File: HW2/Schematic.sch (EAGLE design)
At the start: 3 parts

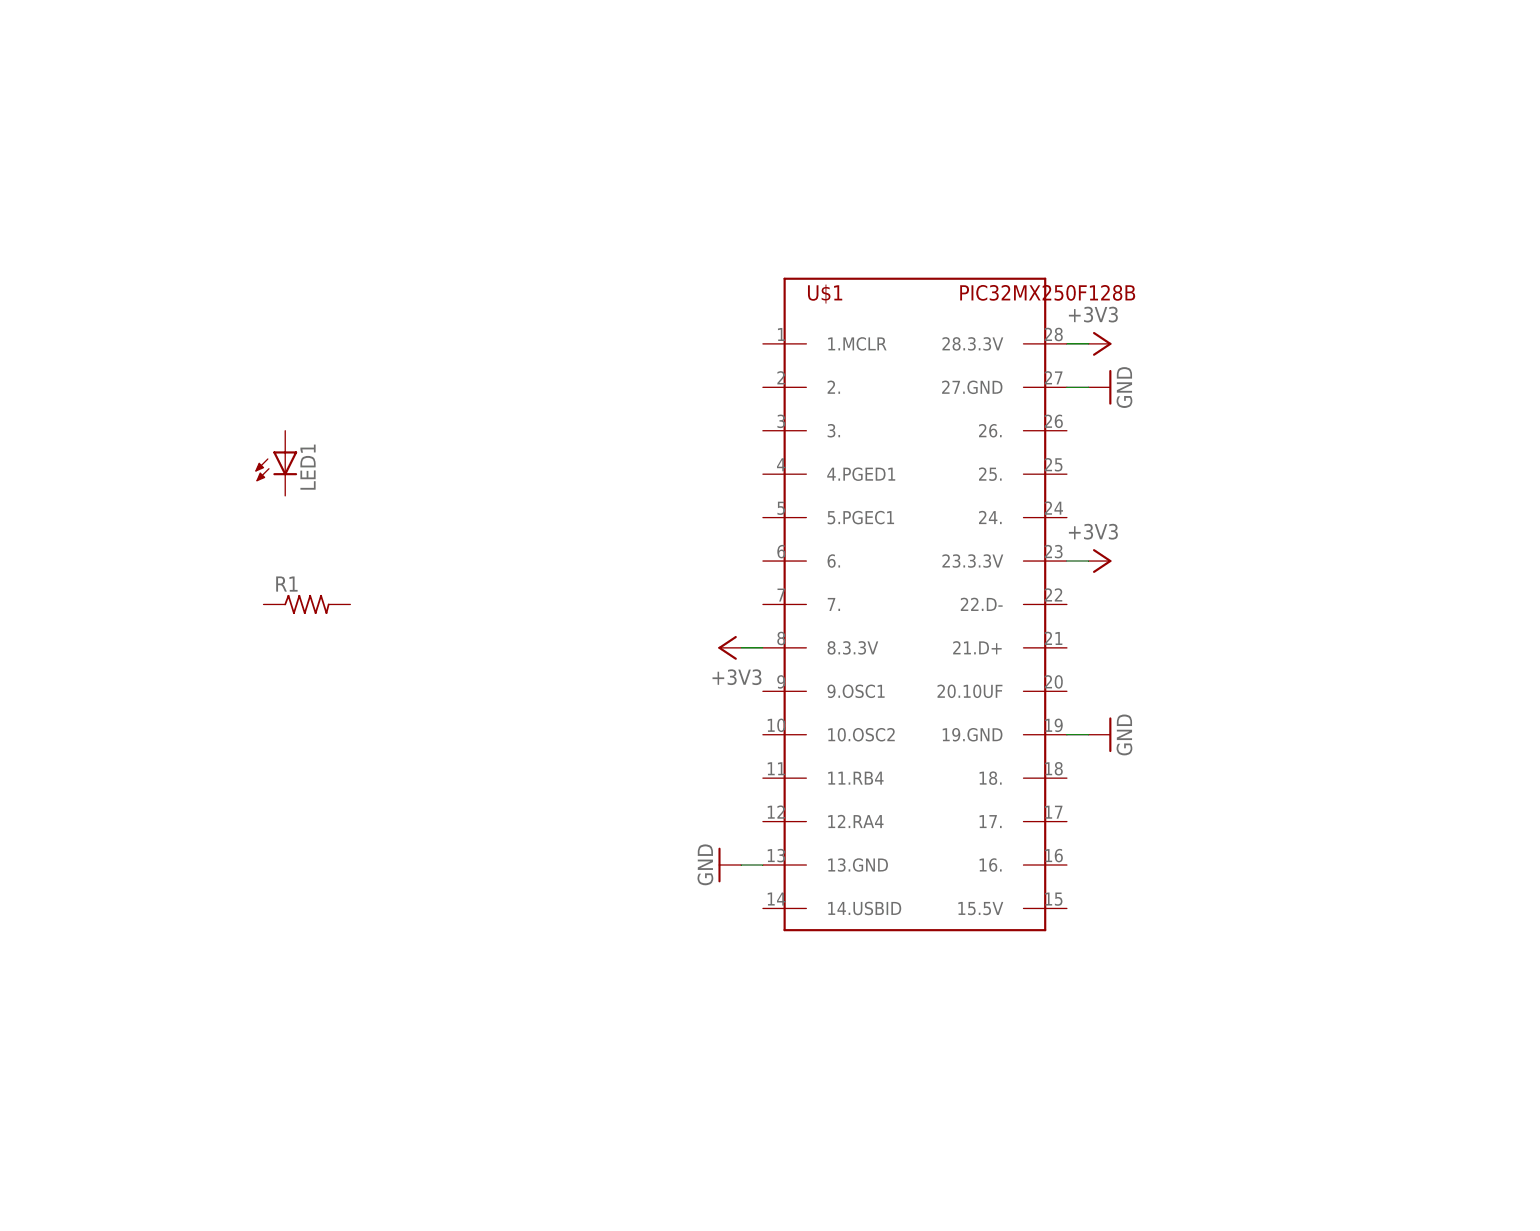
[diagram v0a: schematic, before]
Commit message: schematic done
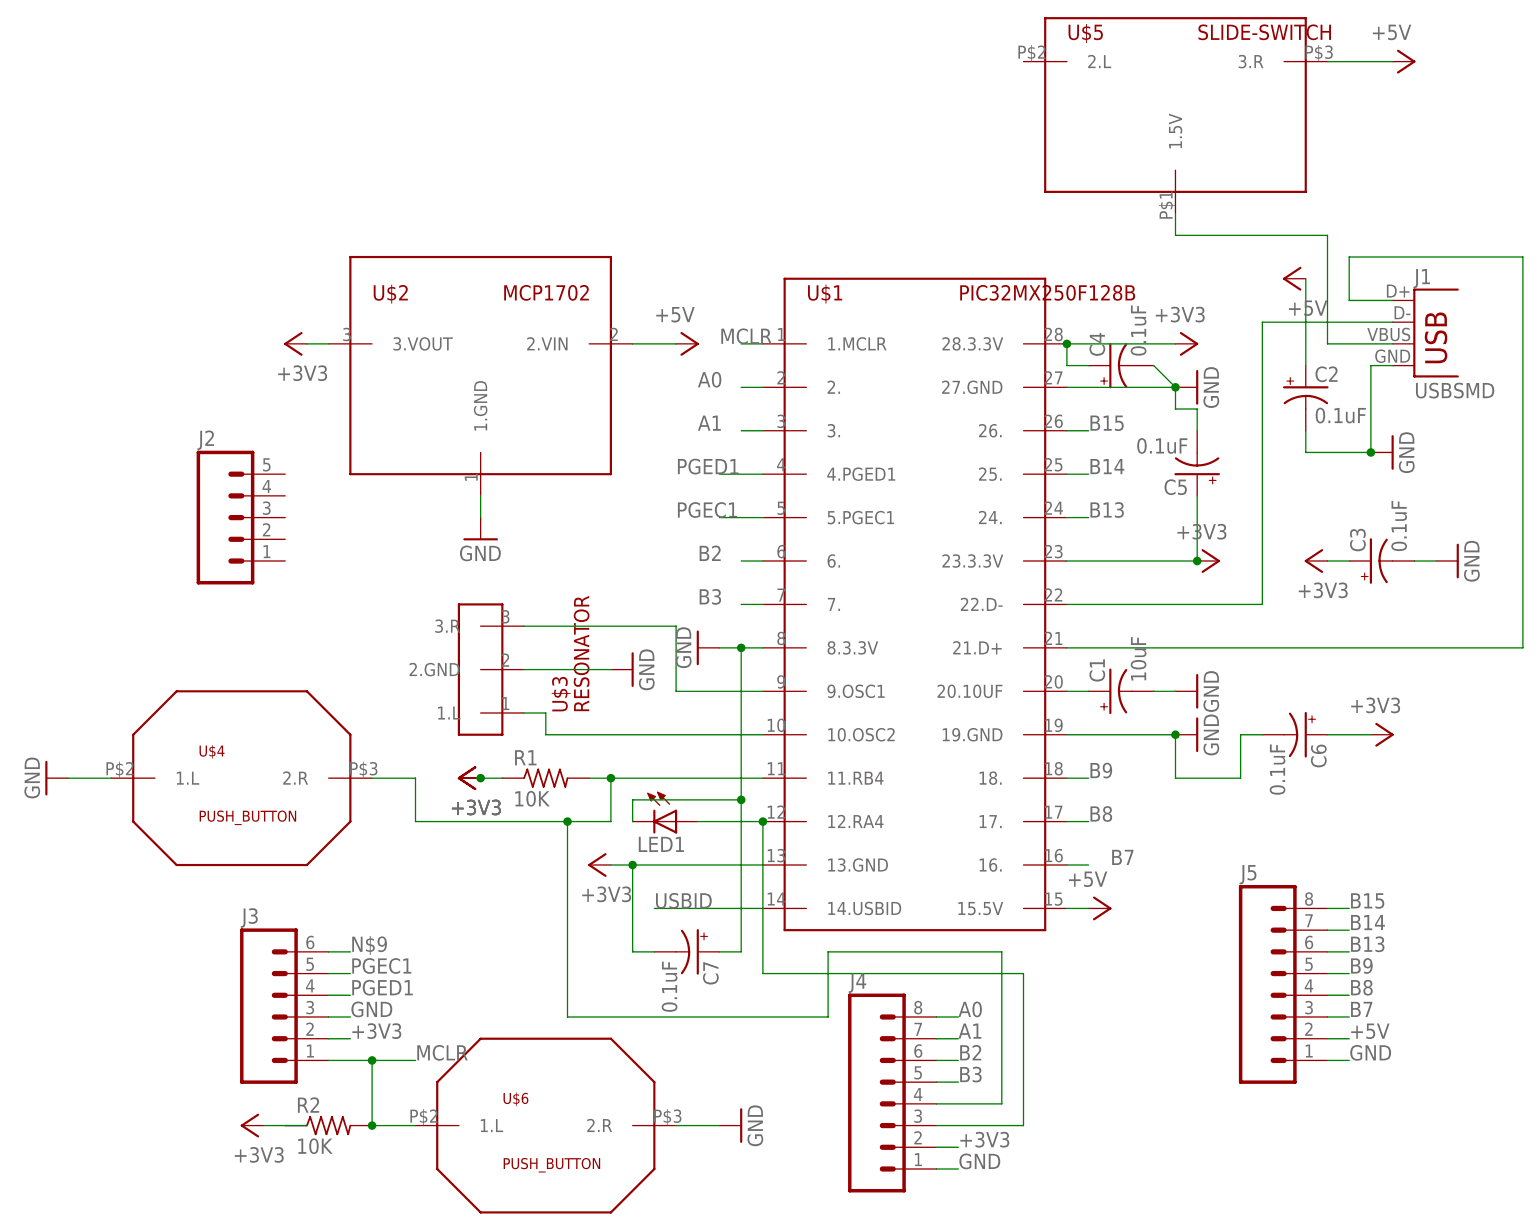
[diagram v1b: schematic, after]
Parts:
- added C1: 10uF, pic32_library:CPOL-USE2.5-5
- added C2, C3, C4, C5, C6, C7: 0.1uF, pic32_library:CPOL-USE2.5-5
- added J1: USBSMD, pic32_library:USBSMD
- added J2: (no value), pic32_library:M05PTH
- added J3: (no value), pic32_library:M06SILK_FEMALE_PTH
- added J4, J5: (no value), pic32_library:M08SILK_FEMALE_PTH
- added R2: 10K, pic32_library:R-US_0207/10
- added U$2: MCP1702, pic32_library:MCP1702
- added U$3: RESONATOR, pic32_library:RESONATOR
- added U$4, U$6: PUSH_BUTTON, pic32_library:PUSH_BUTTON
- added U$5: SLIDE-SWITCH, pic32_library:SLIDE-SWITCH
- R1: value (none) -> 10K
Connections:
- new net +5V: C2.+, J5.2, U$1.15.5V, U$2.2.VIN, U$5.3.R
- new net A0: J4.8, U$1.2.
- new net A1: J4.7, U$1.3.
- new net A4: J4.3, LED1.A, U$1.12.RA4
- new net B13: J5.6, U$1.24.
- new net B14: J5.7, U$1.25.
- new net B15: J5.8, U$1.26.
- new net B2: J4.6, U$1.6.
- new net B3: J4.5, U$1.7.
- new net B4: J4.4, R1.2, U$1.11.RB4, U$4.2.R
- new net B7: J5.3, U$1.16.
- new net B8: J5.4, U$1.17.
- new net B9: J5.5, U$1.18.
- new net MCLR: J3.1, R2.2, U$1.1.MCLR, U$6.1.L
- new net N$1: C1.+, U$1.20.10UF
- new net N$2: J1.D-, U$1.22.D-
- new net N$3: J1.D+, U$1.21.D+
- new net N$4: U$1.9.OSC1, U$3.3.R
- new net N$5: U$1.10.OSC2, U$3.1.L
- new net N$6: J1.VBUS, U$5.1.5V
- new net N$9: J3.6
- new net PGEC1: J3.5, U$1.5.PGEC1
- new net PGED1: J3.4, U$1.4.PGED1
- new net USBID: U$1.14.USBID
- net +3V3: now also C3.+, C4.+, C5.+, C6.+, C7.-, J3.2, J4.2, R1.1, U$1.13.GND, U$2.3.VOUT; no longer U$1.8.3.3V
- net GND: now also C1.-, C2.-, C3.-, C4.-, C5.-, C6.-, C7.+, J1.GND, J3.3, J4.1, J5.1, LED1.C, U$1.8.3.3V, U$2.1.GND, U$3.2.GND, U$4.1.L, U$6.2.R; no longer U$1.13.GND
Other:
- moved on the sheet: LED1, R1
